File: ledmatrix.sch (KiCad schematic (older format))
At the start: 89 parts, among them U58 sled1735

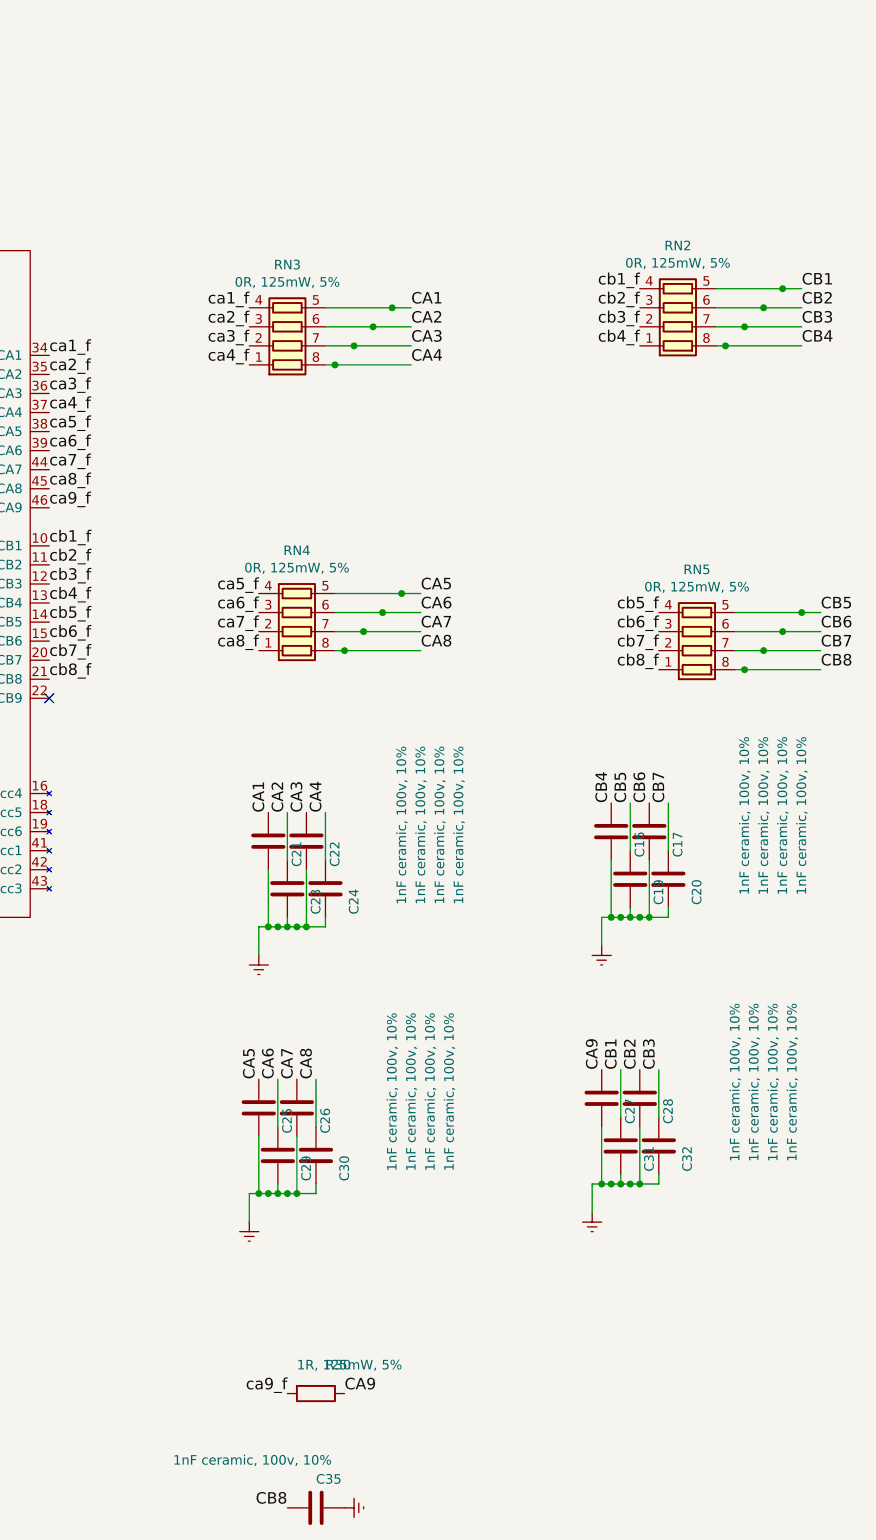
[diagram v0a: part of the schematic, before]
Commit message: cleanup
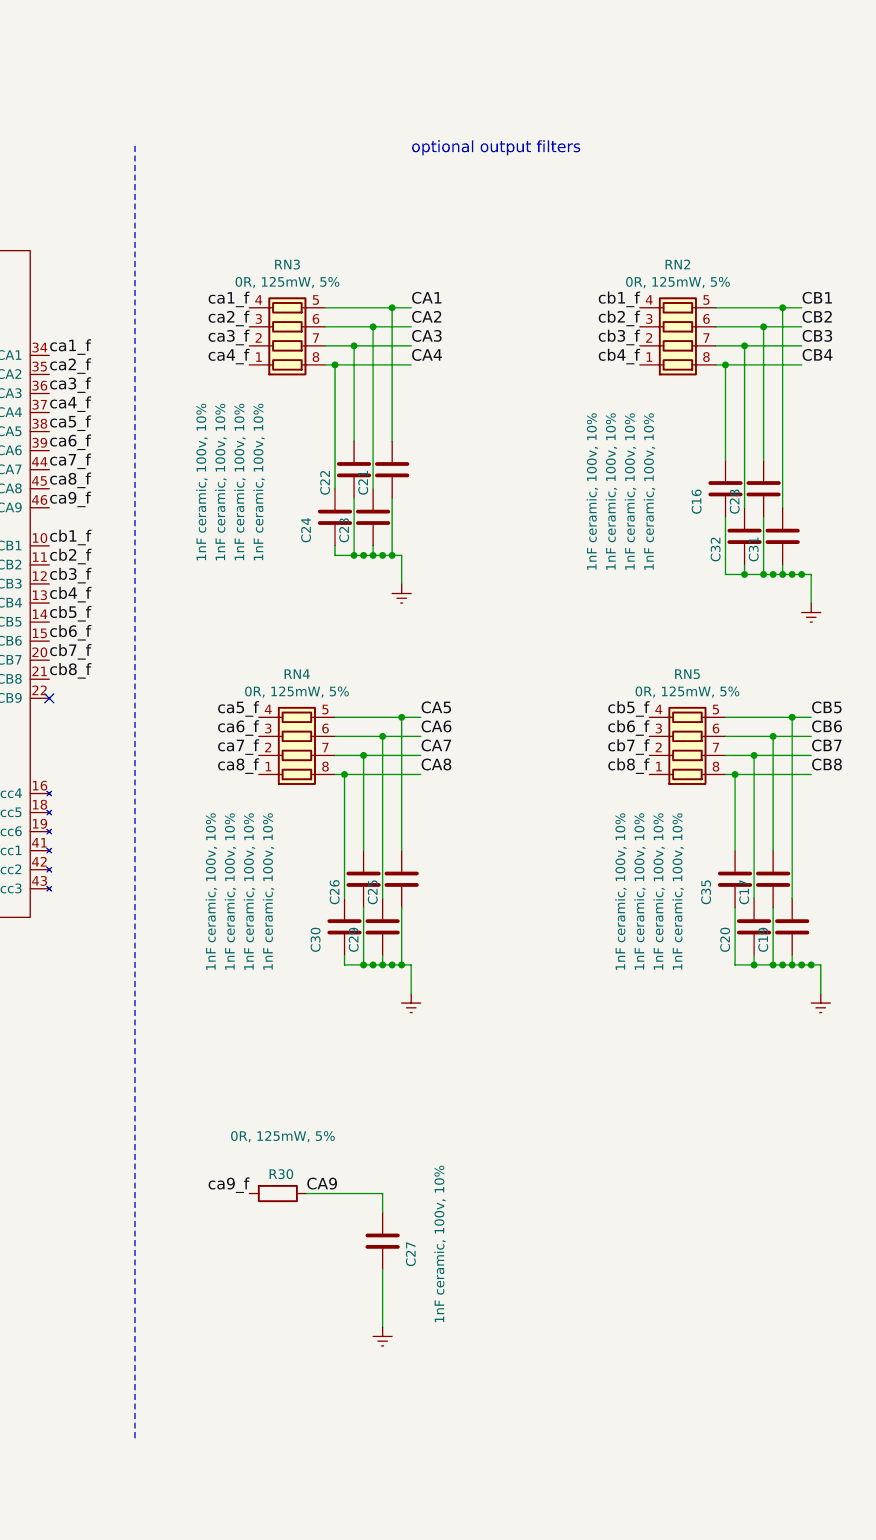
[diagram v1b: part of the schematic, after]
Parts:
- R30: value 1R, 125mW, 5% -> 0R, 125mW, 5%
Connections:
- wire segments 104 -> 115
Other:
- note added: "optional output filters\n"
- moved on the sheet: C16, C17, C19, C20, C21, C22, C23, C24, C25, C26, C27, C28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
